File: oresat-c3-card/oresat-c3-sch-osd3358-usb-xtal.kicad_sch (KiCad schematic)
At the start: 38 parts, among them U1 OSD3358-1G-ISM, U11 RCLAMP0504FB, Y1 ECS-240-12-30BQ-AEN-TR, Y2 ABS07-32.768KHZ-T

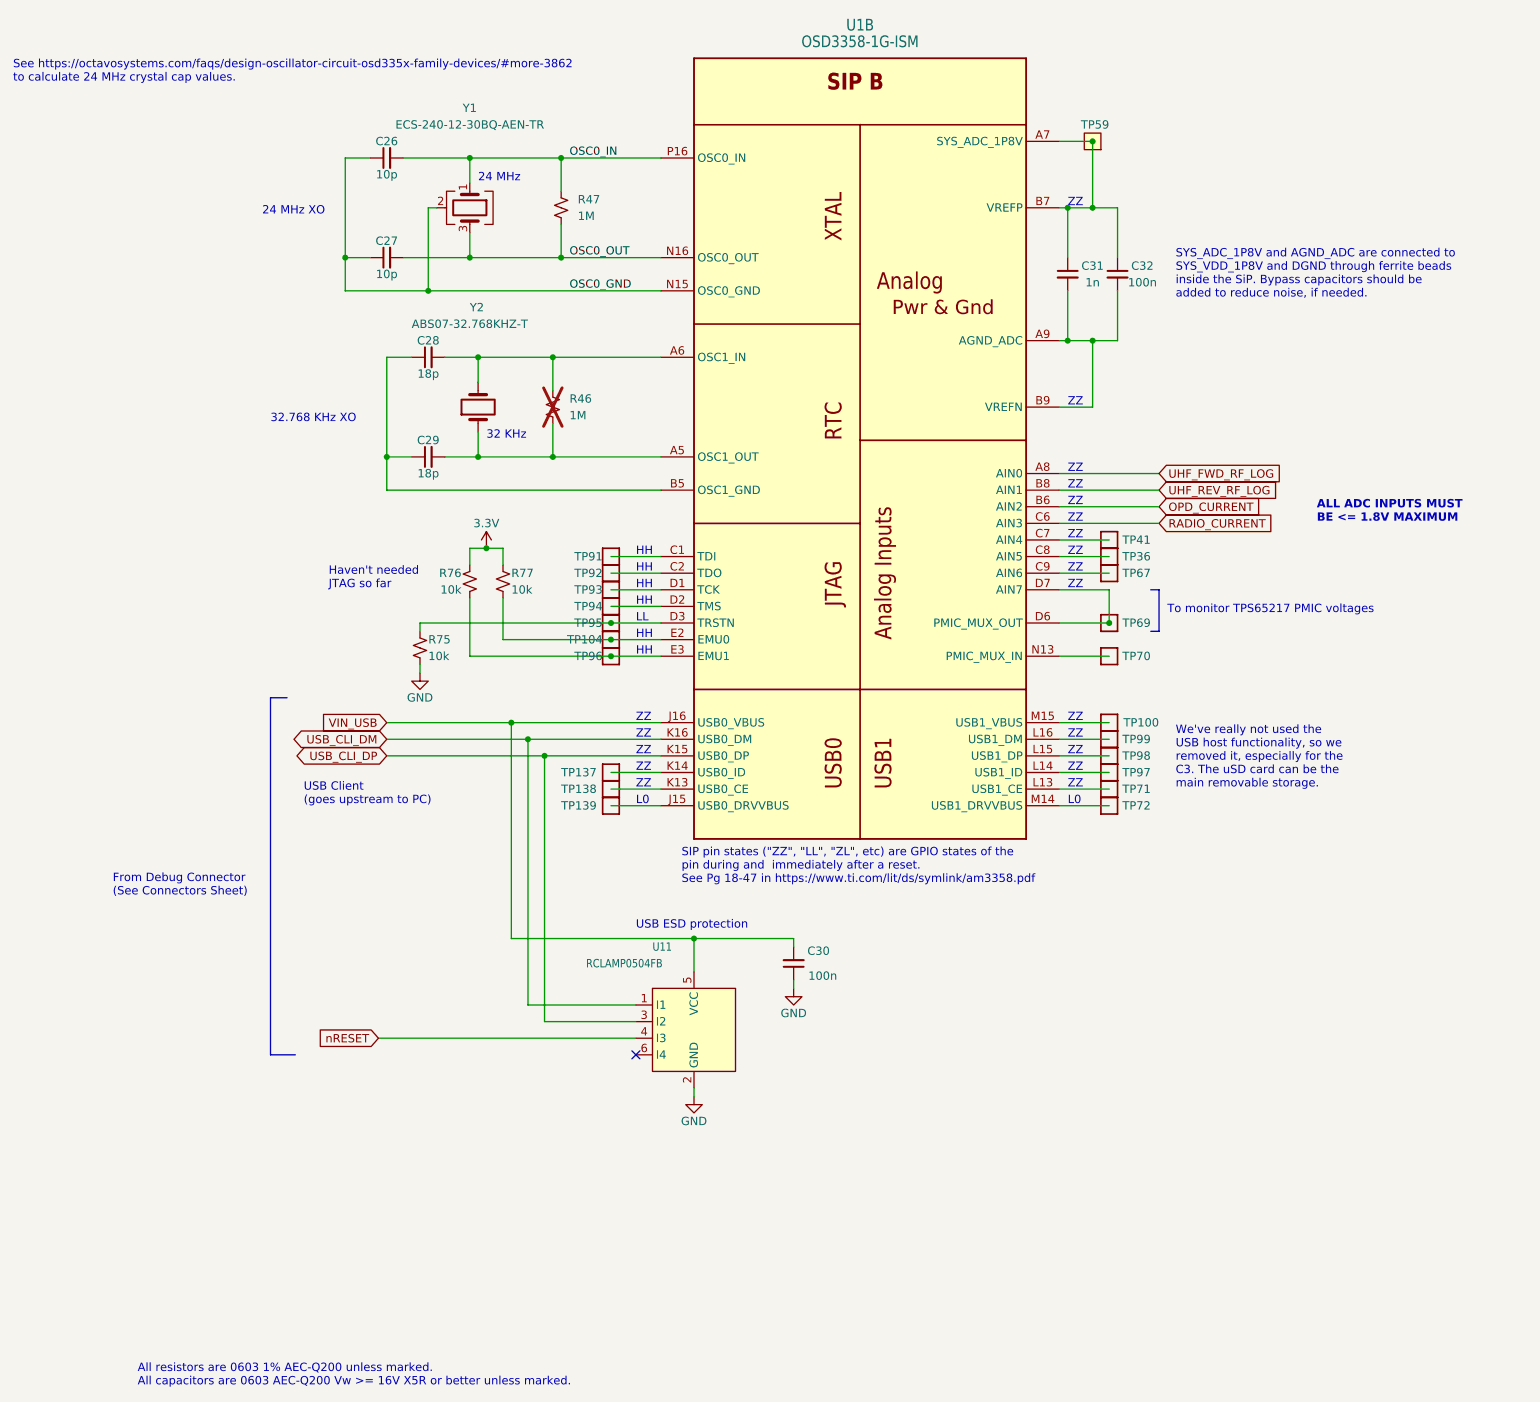
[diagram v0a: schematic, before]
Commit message: Changed to hierarchy view
Updated schematic to hierarchy view, replaced couple of footprints on pcb and schematic symbols. Deleted connectors sheet.
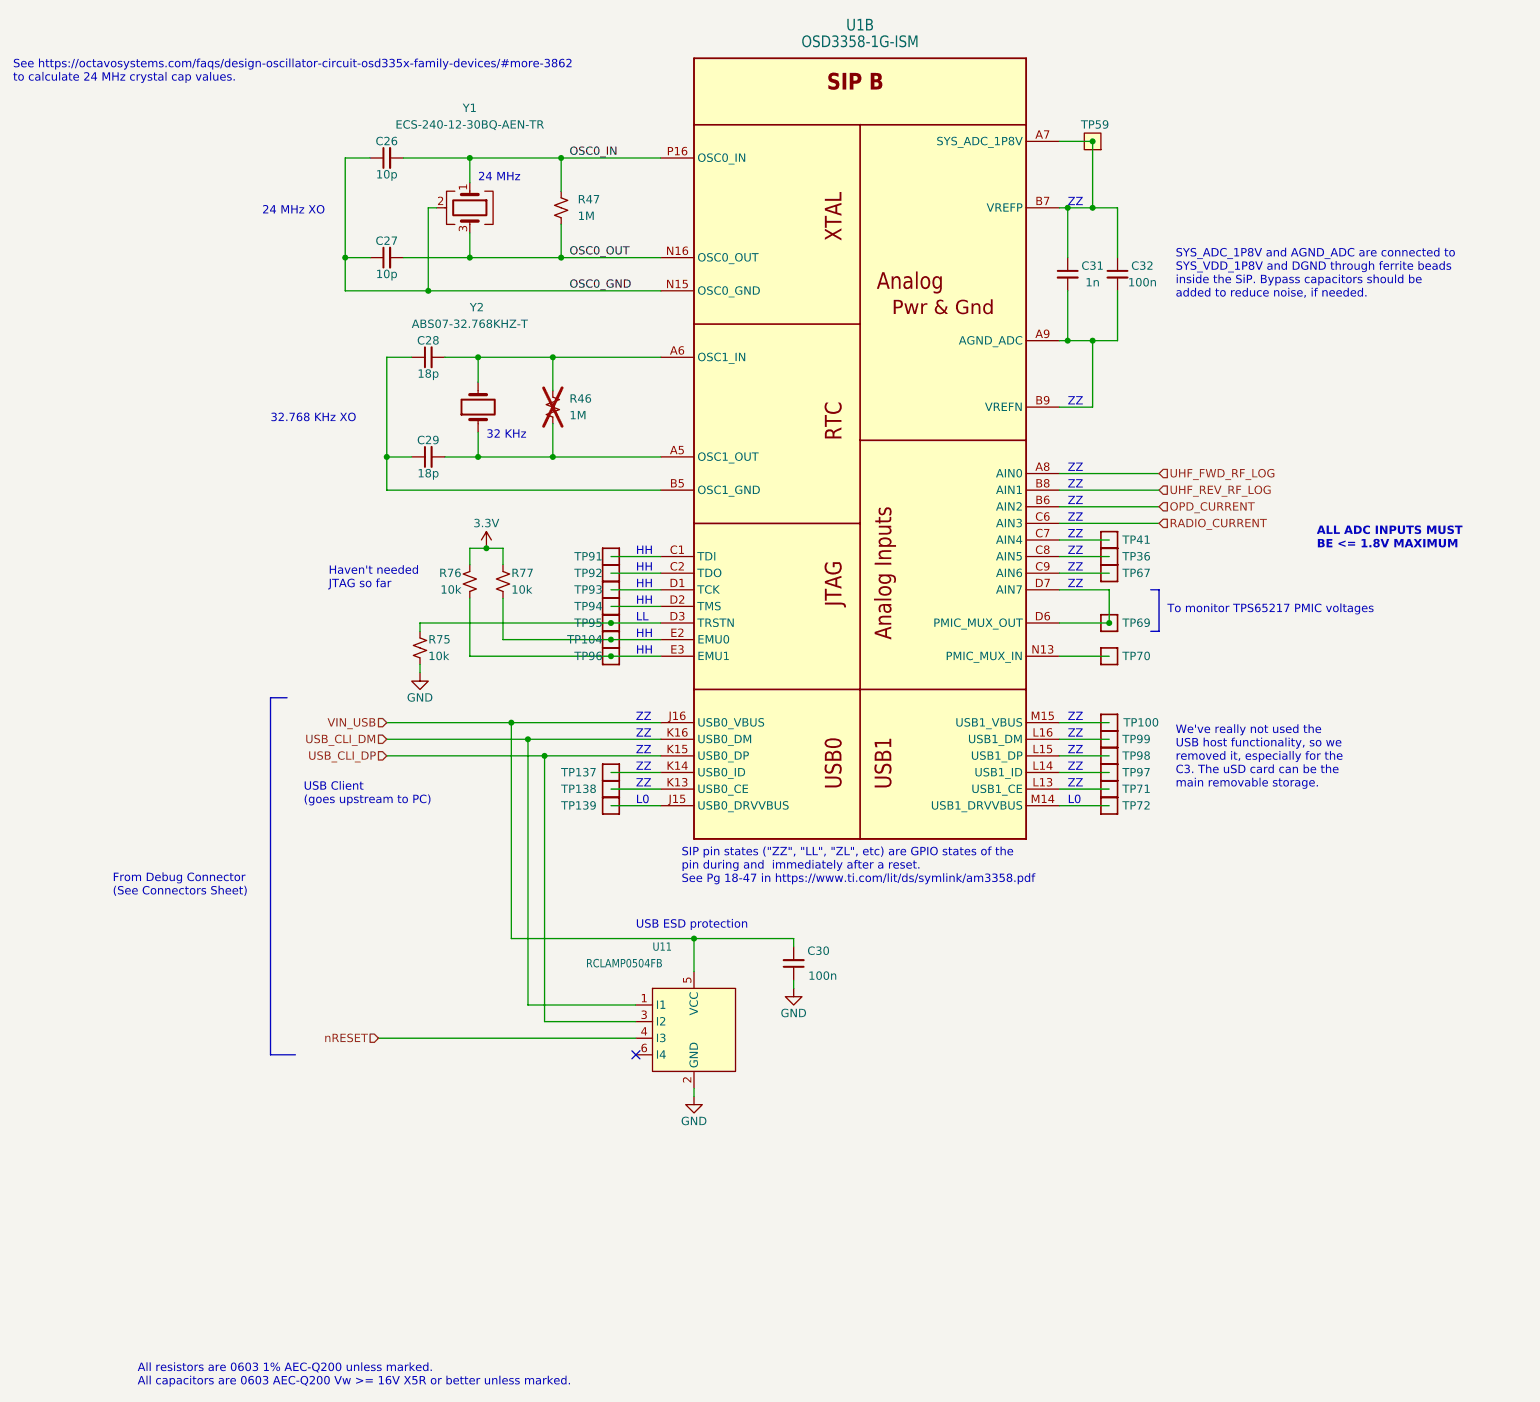
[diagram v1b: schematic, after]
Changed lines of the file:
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@@
 	(text "ALL ADC INPUTS MUST\nBE <= 1.8V MAXIMUM"
 		(exclude_from_sim no)
-		(at 295.91 129.54 0)
+		(at 295.91 133.604 0)
 		(effects
 			(font
@@
 		)
 	)
-	(global_label "USB_CLI_DP"
-		(shape bidirectional)
-		(at 153.67 165.1 180)
+	(hierarchical_label "VIN_USB"
+		(shape input)
+		(at 153.67 160.02 180)
 		(effects
 			(font
@@
 			(justify right)
 		)
-		(property "Intersheetrefs" "${INTERSHEET_REFS}"
-			(at 139.7 165.1 0)
-			(show_name no)
-			(do_not_autoplace no)
-			(effects
-				(font
-					(size 1.27 1.27)
-				)
-				(justify right)
-			)
-		)
-	)
-	(global_label "OPD_CURRENT"
+	)
+	(hierarchical_label "nRESET"
+		(shape input)
+		(at 152.4 208.28 180)
+		(effects
+			(font
+				(size 1.27 1.27)
+			)
+			(justify right)
+		)
+	)
+	(hierarchical_label "OPD_CURRENT"
 		(shape input)
 		(at 271.78 127 0)
-		(fields_autoplaced yes)
 		(effects
 			(font
@@
 			(justify left)
 		)
-		(property "Intersheetrefs" "${INTERSHEET_REFS}"
-			(at 288.1115 127 0)
-			(show_name no)
-			(do_not_autoplace no)
-			(effects
-				(font
-					(size 1.27 1.27)
-				)
-				(justify left)
-			)
-		)
-	)
-	(global_label "nRESET"
+	)
+	(hierarchical_label "USB_CLI_DP"
 		(shape input)
-		(at 152.4 208.28 180)
+		(at 153.67 165.1 180)
 		(effects
 			(font
@@
 			(justify right)
 		)
-		(property "Intersheetrefs" "${INTERSHEET_REFS}"
-			(at 142.24 208.28 0)
-			(show_name no)
-			(do_not_autoplace no)
-			(effects
-				(font
-					(size 1.27 1.27)
-				)
-				(justify right)
-			)
-		)
-	)
-	(global_label "USB_CLI_DM"
-		(shape bidirectional)
-		(at 153.67 162.56 180)
-		(effects
-			(font
-				(size 1.27 1.27)
-			)
-			(justify right)
-		)
-		(property "Intersheetrefs" "${INTERSHEET_REFS}"
-			(at 139.7 162.56 0)
-			(show_name no)
-			(do_not_autoplace no)
-			(effects
-				(font
-					(size 1.27 1.27)
-				)
-				(justify right)
-			)
-		)
-	)
-	(global_label "UHF_FWD_RF_LOG"
+	)
+	(hierarchical_label "UHF_FWD_RF_LOG"
 		(shape input)
 		(at 271.78 121.92 0)
-		(fields_autoplaced yes)
 		(effects
 			(font
@@
 			(justify left)
 		)
-		(property "Intersheetrefs" "${INTERSHEET_REFS}"
-			(at 291.1354 121.92 0)
-			(show_name no)
-			(do_not_autoplace no)
-			(effects
-				(font
-					(size 1.27 1.27)
-				)
-				(justify left)
-			)
-		)
-	)
-	(global_label "UHF_REV_RF_LOG"
+	)
+	(hierarchical_label "USB_CLI_DM"
+		(shape input)
+		(at 153.67 162.56 180)
+		(effects
+			(font
+				(size 1.27 1.27)
+			)
+			(justify right)
+		)
+	)
+	(hierarchical_label "RADIO_CURRENT"
+		(shape input)
+		(at 271.78 129.54 0)
+		(effects
+			(font
+				(size 1.27 1.27)
+			)
+			(justify left)
+		)
+	)
+	(hierarchical_label "UHF_REV_RF_LOG"
 		(shape input)
 		(at 271.78 124.46 0)
-		(fields_autoplaced yes)
 		(effects
 			(font
@@
 			(justify left)
 		)
-		(property "Intersheetrefs" "${INTERSHEET_REFS}"
-			(at 290.833 124.46 0)
-			(show_name no)
-			(do_not_autoplace no)
-			(effects
-				(font
-					(size 1.27 1.27)
-				)
-				(justify left)
-			)
-		)
-	)
-	(global_label "VIN_USB"
-		(shape input)
-		(at 153.67 160.02 180)
-		(fields_autoplaced yes)
-		(effects
-			(font
-				(size 1.27 1.27)
-			)
-			(justify right)
-		)
-		(property "Intersheetrefs" "${INTERSHEET_REFS}"
-			(at 143.4555 159.9406 0)
-			(show_name no)
-			(do_not_autoplace no)
-			(effects
-				(font
-					(size 1.27 1.27)
-				)
-				(justify right)
-			)
-		)
-	)
-	(global_label "RADIO_CURRENT"
-		(shape input)
-		(at 271.78 129.54 0)
-		(fields_autoplaced yes)
-		(effects
-			(font
-				(size 1.27 1.27)
-			)
-			(justify left)
-		)
-		(property "Intersheetrefs" "${INTERSHEET_REFS}"
-			(at 289.8049 129.54 0)
-			(show_name no)
-			(do_not_autoplace no)
-			(effects
-				(font
-					(size 1.27 1.27)
-				)
-				(justify left)
-			)
-		)
-	)
+	)
